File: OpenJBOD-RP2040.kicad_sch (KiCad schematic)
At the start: 63 parts, among them J1 ATX-24, J2 Bus_PCI_Express_x1, J3 Conn_02x02_Counter_Clockwise, J4 UART, J5 USB_C_Receptacle_USB2.0_16P, J9 TEMP1, Q1 MMBT3904, Q2 MMBT3904, SW1 TC-6615-6-260G, SW2 TC-6615-6-260G, SW3 TC-6615-6-260G, U1 RP2040, U2 AMS1117-3.3, U3 W25Q128JVS, U5 74LVC1G02, U7 74LVC1G02, U8 DS18B20U, Y1 X322512MSB4SI

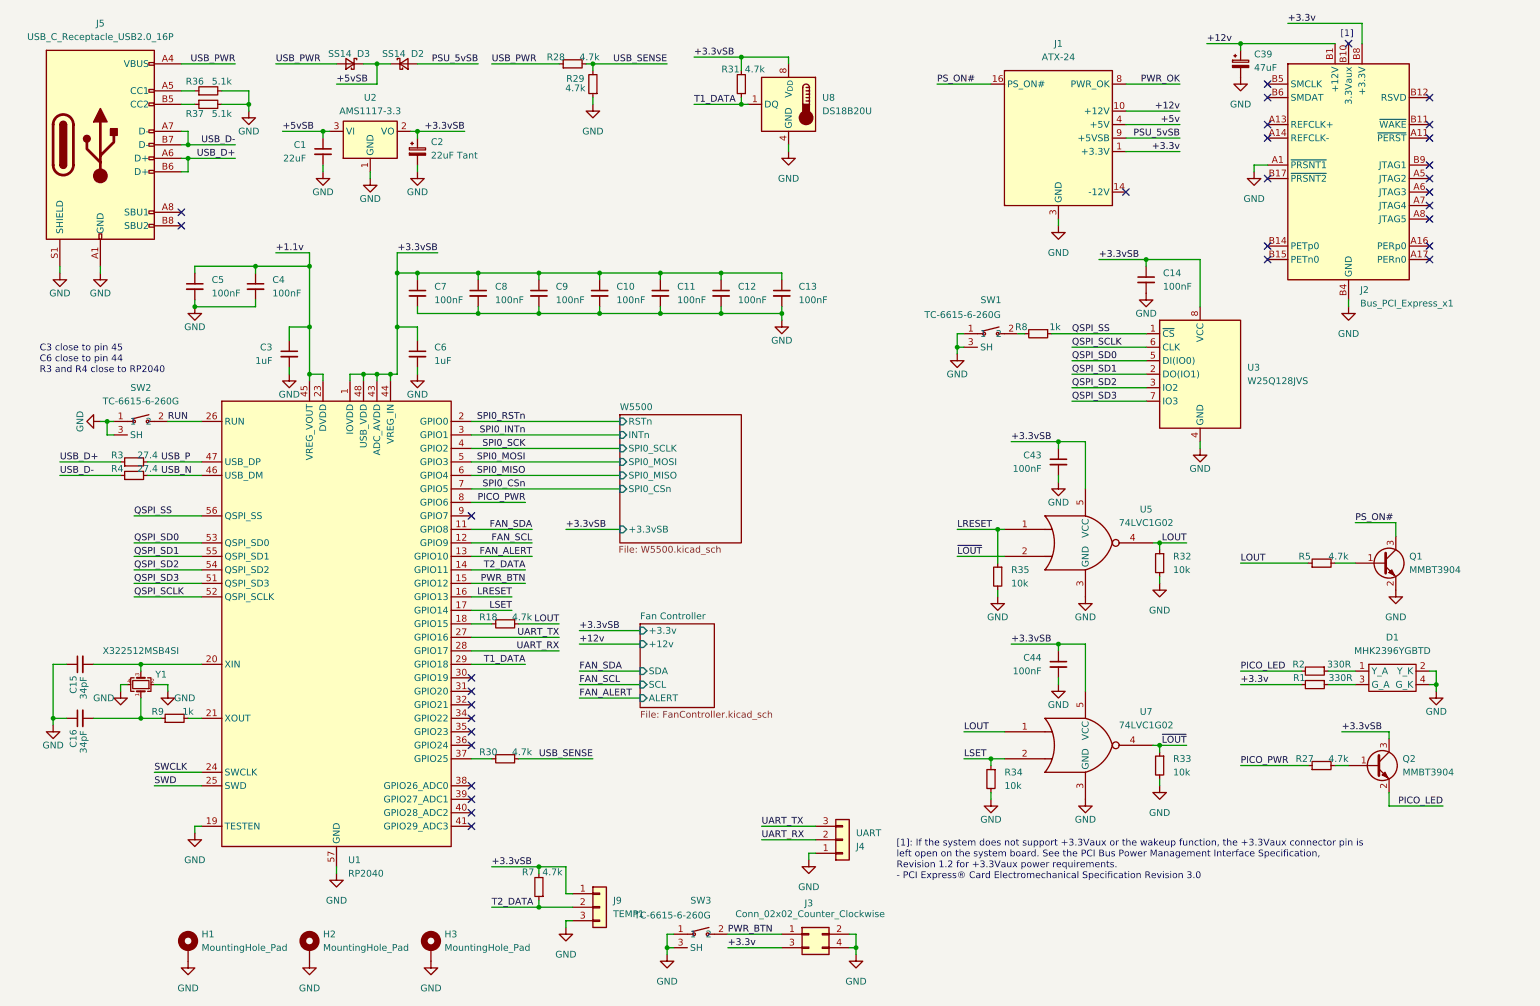
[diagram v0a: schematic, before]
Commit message: schematic cleanup
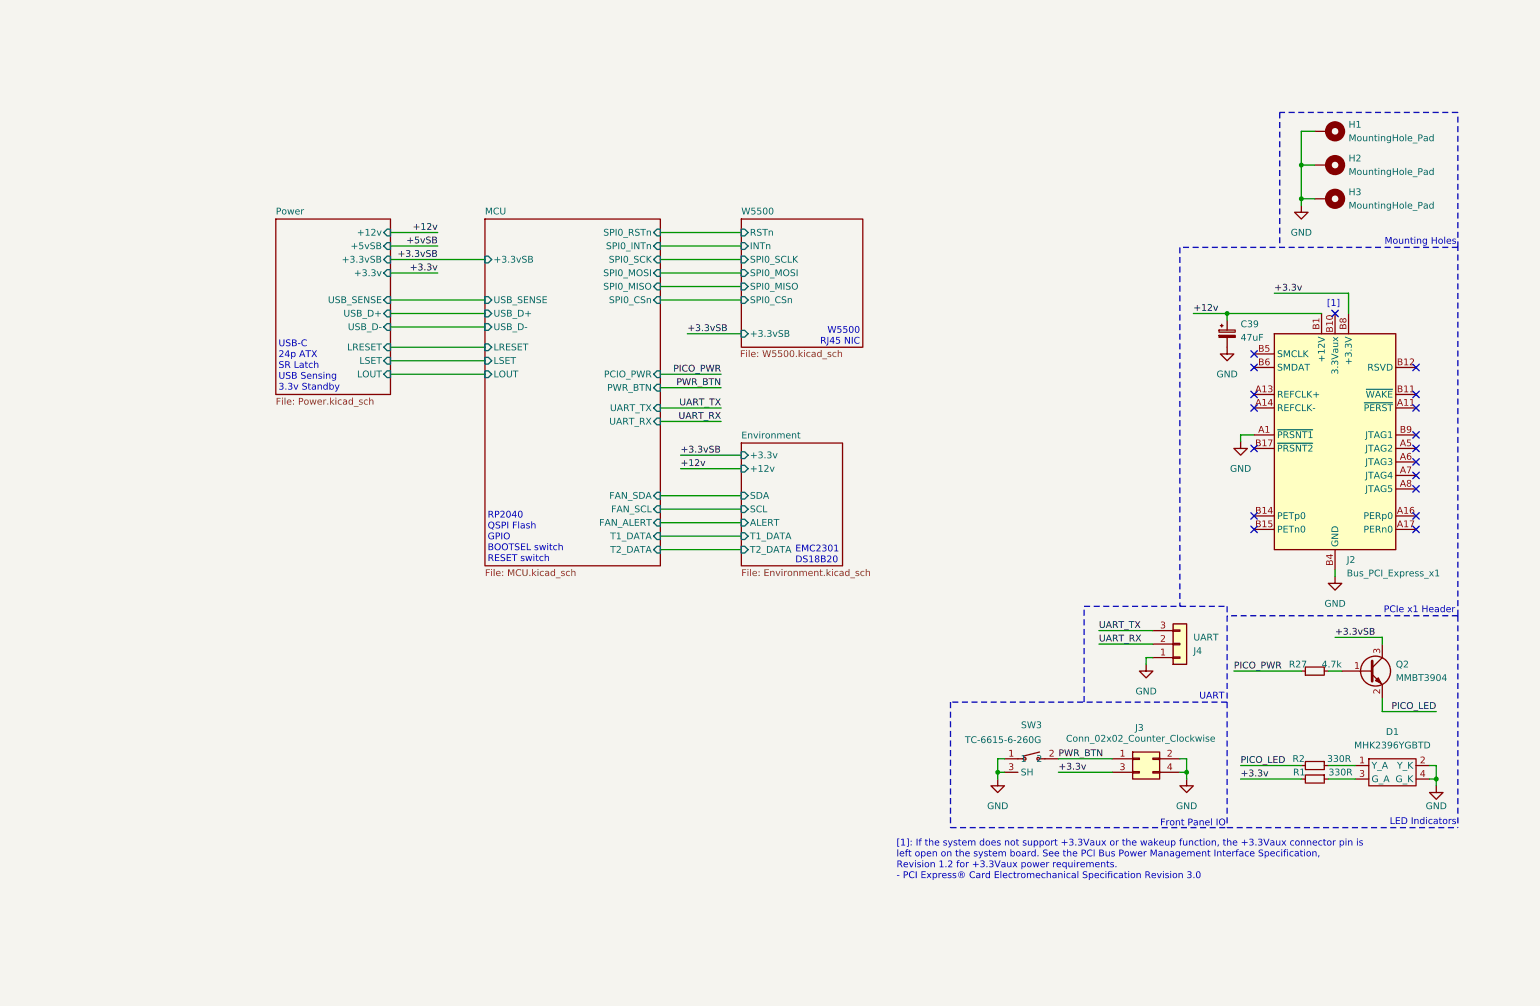
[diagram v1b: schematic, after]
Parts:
- removed C1: 22uF, Capacitor_SMD:C_1206_3216Metric, symbol Device:C_Small
- removed C10, C11, C12, C13, C14, C4, C43, C44, C5, C7, C8, C9: 100nF, Capacitor_SMD:C_0402_1005Metric, symbol Device:C_Small
- removed C15, C16: 34pF, Capacitor_SMD:C_0603_1608Metric, symbol Device:C_Small
- removed C2: 22uF Tant, Capacitor_Tantalum_SMD:CP_EIA-3216-18_Kemet-A, symbol Device:C_Polarized_Small
- removed C3, C6: 1uF, Capacitor_SMD:C_0402_1005Metric, symbol Device:C_Small
- removed D2, D3: SS14, Diode_SMD:D_SMA, symbol Device:D_Schottky_Small
- removed J1: ATX-24, OpenJBOD_Library:CONN-TH_M4202V-2X12P, symbol Connector:ATX-24
- removed J5: USB_C_Receptacle_USB2.0_16P, OpenJBOD_Library:USB-C-SMD_TYPE-C16PIN, symbol Connector:USB_C_Receptacle_USB2.0_16P
- removed J9: TEMP1, Connector_PinHeader_2.54mm:PinHeader_1x03_P2.54mm_Vertical, symbol Connector_Generic:Conn_01x03
- removed Q1: MMBT3904, Package_TO_SOT_SMD:SOT-23, symbol Transistor_BJT:MMBT3904
- removed R18, R28, R29, R30, R31, R5, R7: 4.7k, Resistor_SMD:R_0402_1005Metric, symbol Device:R_Small
- removed R3, R4: 27.4, Resistor_SMD:R_0402_1005Metric, symbol Device:R_Small
- removed R32, R33, R34, R35: 10k, Capacitor_SMD:C_0402_1005Metric, symbol Device:R_Small
- removed R36, R37: 5.1k, Capacitor_SMD:C_0402_1005Metric, symbol Device:R_Small
- removed R8, R9: 1k, Resistor_SMD:R_0402_1005Metric, symbol Device:R_Small
- removed SW1, SW2: TC-6615-6-260G, OpenJBOD_Library:KEY-TH_TC-6615-6-160G, symbol OpenJBOD:TC-6615-6-260G
- removed U1: RP2040, Package_DFN_QFN:QFN-56-1EP_7x7mm_P0.4mm_EP3.2x3.2mm, symbol MCU_RaspberryPi:RP2040
- removed U2: AMS1117-3.3, Package_TO_SOT_SMD:SOT-223-3_TabPin2, symbol Regulator_Linear:AMS1117-3.3
- removed U3: W25Q128JVS, Package_SO:SOIC-8_5.23x5.23mm_P1.27mm, symbol Memory_Flash:W25Q128JVS
- removed U5, U7: 74LVC1G02, Package_TO_SOT_SMD:SOT-353_SC-70-5, symbol 74xGxx:74LVC1G02
- removed U8: DS18B20U, Package_SO:MSOP-8_3x3mm_P0.65mm, symbol Sensor_Temperature:DS18B20U
- removed Y1: X322512MSB4SI, Crystal:Crystal_SMD_3225-4Pin_3.2x2.5mm, symbol Device:Crystal_GND24_Small
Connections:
- no-connect marks 32 -> 18
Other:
- sheet Fan Controller renamed Environment
- added sheet MCU (MCU.kicad_sch)
- added sheet Power (Power.kicad_sch)
- sheet Environment: file FanController.kicad_sch -> Environment.kicad_sch
- sheet Environment ports: added T1_DATA, T2_DATA; removed none
- note added: "EMC2301 DS18B20"
- note added: "Front Panel IO"
- note added: "LED Indicators"
- note added: "Mounting Holes"
- note added: "PCIe x1 Header"
- note added: "RP2040 QSPI Flash GPIO BOOTSEL switch RESET switch"
- note added: "UART"
- note added: "USB-C 24p ATX SR Latch USB Sensing 3.3v Standby"
- note added: "W5500 RJ45 NIC"
- note removed: "C3 close to pin 45 C6 close to pin 44 R3 and R4 close to RP2040"
- moved on the sheet: C39, D1, H1, H2, H3, J2, J3, J4, Q2, R1, R2, R27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
